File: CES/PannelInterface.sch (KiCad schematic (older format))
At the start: 26 parts, among them U701 BS1, U702 BS2, U703 74HC04, U704 74HC04, U705 74HC04, U706 74HC04, U707 74HC04, U708 74HC04, U709 74HC04, U710 74HC04

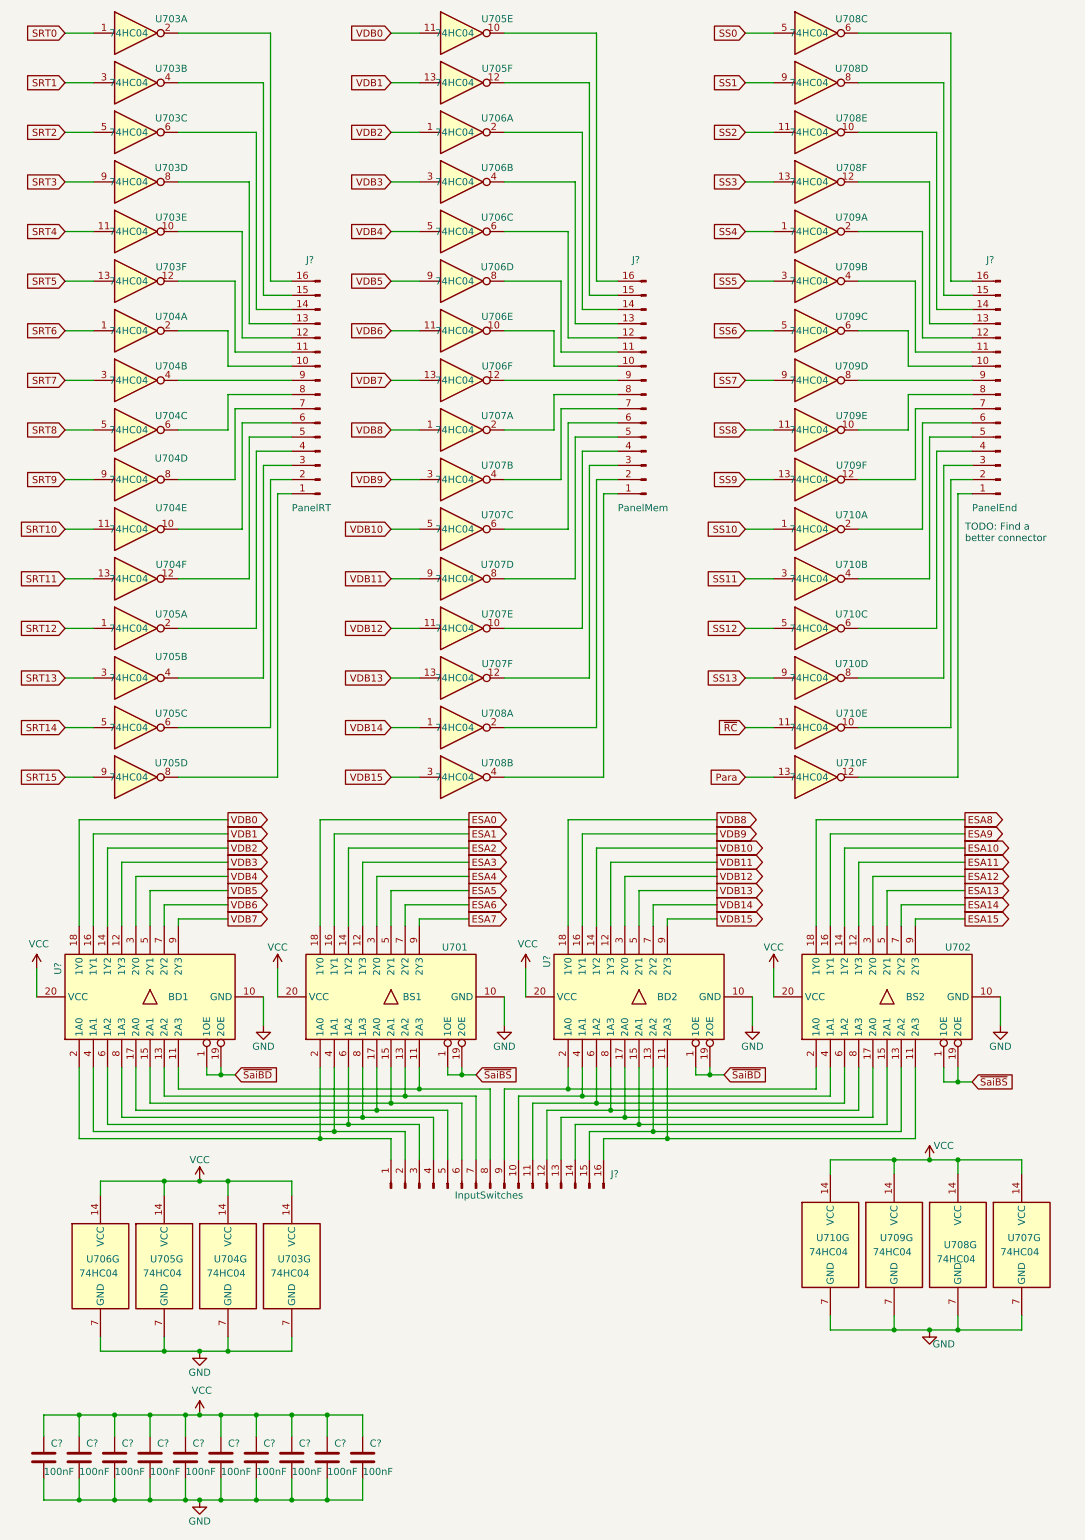
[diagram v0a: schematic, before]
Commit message: Registers
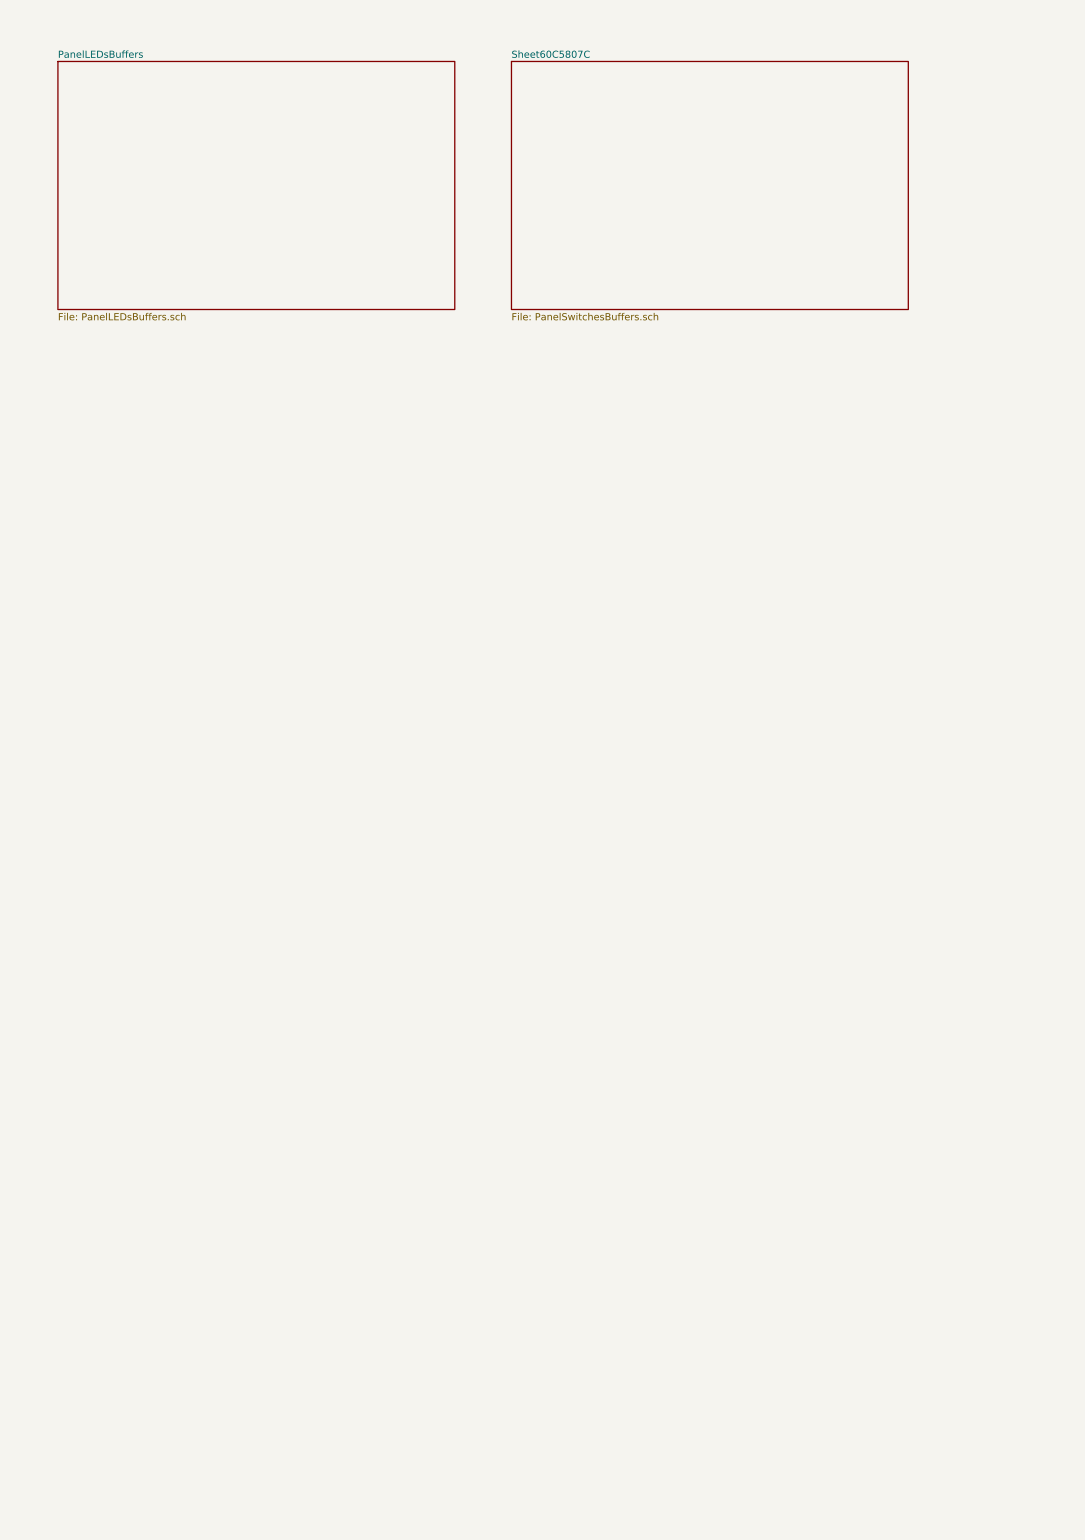
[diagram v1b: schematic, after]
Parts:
- removed C? (x10): 100nF, symbol Device:C
- removed J?: PanelRT, symbol Connector:Conn_01x16_Male
- removed J?: PanelMem, symbol Connector:Conn_01x16_Male
- removed J?: PanelEnd, symbol Connector:Conn_01x16_Male
- removed J?: InputSwitches, symbol Connector:Conn_01x16_Male
- removed U701: BS1, symbol 74xx:74HC244
- removed U702: BS2, symbol 74xx:74HC244
- removed U703, U704, U705, U706, U707, U708, U709, U710: 74HC04, symbol 74xx:74HC04
- removed U?: BD1, symbol 74xx:74HC244
- removed U?: BD2, symbol 74xx:74HC244
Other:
- note removed: "TODO: Find a \nbetter connector"
